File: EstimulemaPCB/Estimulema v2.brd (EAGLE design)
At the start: 151 x 162 mm, 159 parts, among them IC3 74AC14N, IC4 ISO7240S, J1 JUMPERS12MM, J2 J15MM, J3 J_7MM, J4 JUMPERS5MM, J5 JUMPERS7MM, J6 J7MM, K2 HC-06, Q17 TIP48, Q18 TIP50, Q19 TIP50_TH, Q20 TIP50, Q21 TIP50_TH, Q22 TIP48, Q23 TIP48_TH, Q24 TIP48_TH, Q33 TIP48, Q34 TIP50, Q35 TIP50_TH, Q36 TIP50, Q37 TIP50_TH, Q38 TIP48, Q39 TIP48_TH, Q40 TIP48_TH, X1HV+ CONECTOR_5.08, X2+15- CONECTOR_5.08, X3HV- CONECTOR_5.08

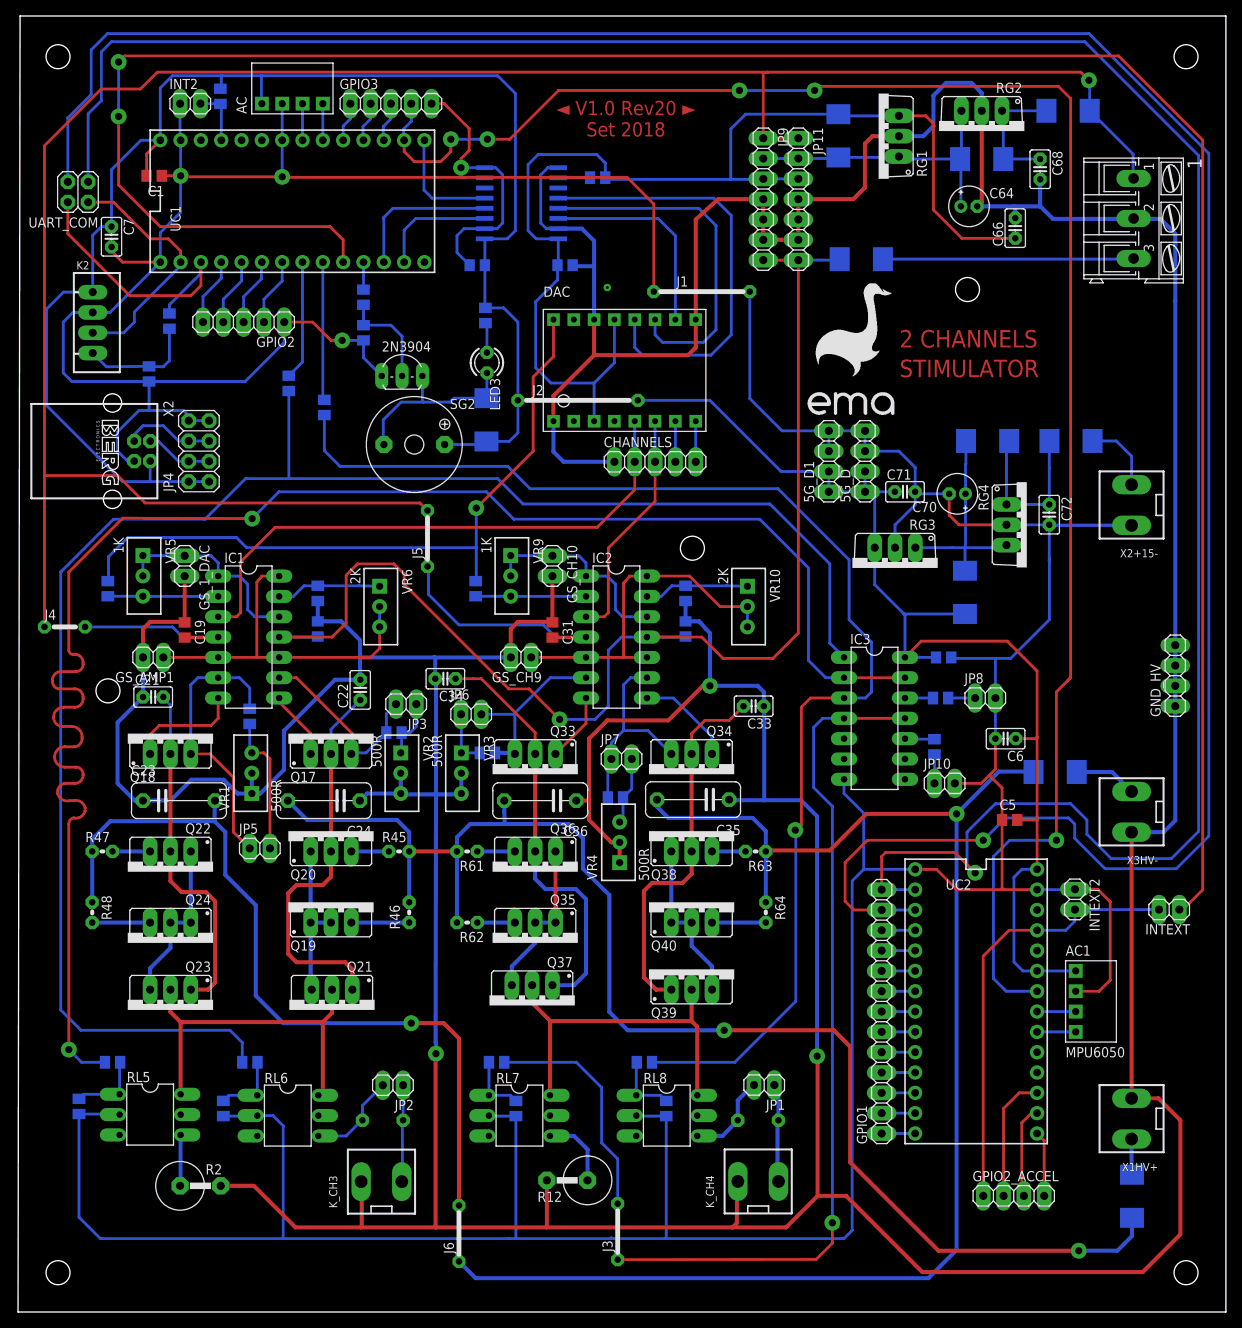
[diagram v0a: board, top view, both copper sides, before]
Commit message: New version eagle 9.2
arreglando algunas cosas
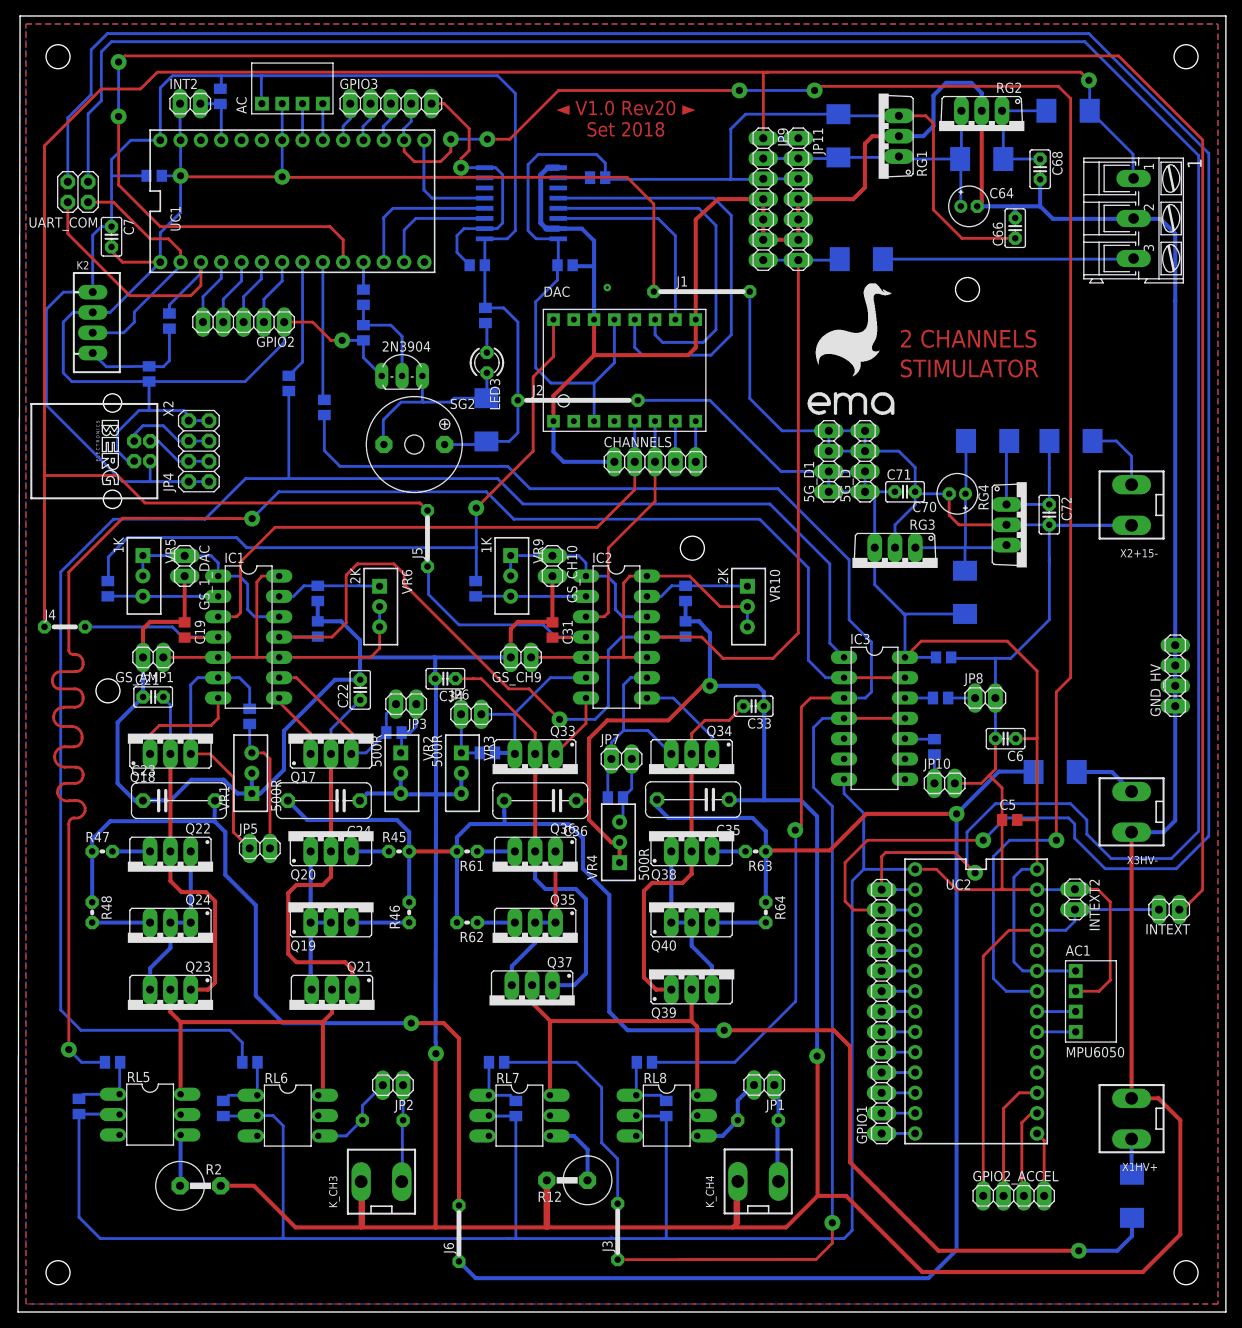
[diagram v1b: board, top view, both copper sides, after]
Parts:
- flipped C1 to the bottom, turned to 0 degrees
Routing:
- net GND_D: track 665.0 -> 669.5 mm
- net +5_D: track 338.5 -> 343.0 mm
- net +8_HV: track 38.6 -> 37.5 mm
- net N$73: track 24.4 -> 23.6 mm
- net N$158: track 22.9 -> 22.3 mm
- net N$145: track 21.1 -> 20.5 mm
- net N$111: track 44.1 -> 43.6 mm
- added copper zone on layer 1, net GND_HV
- added copper zone on layer 16, net GND_HV

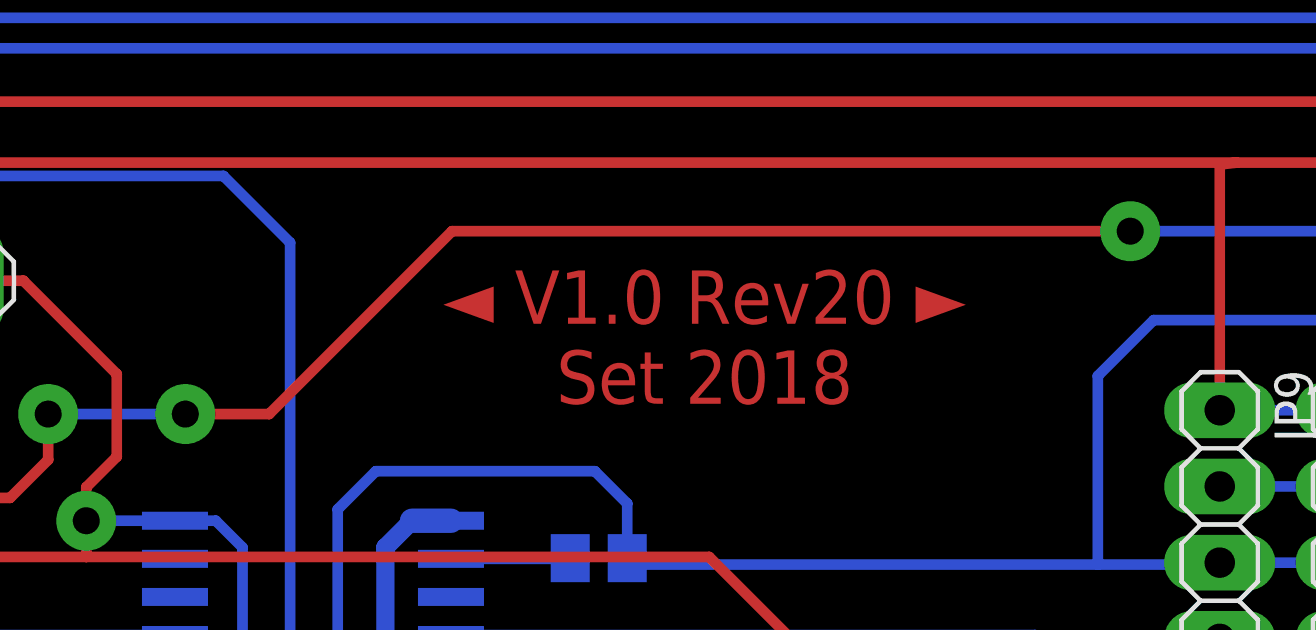
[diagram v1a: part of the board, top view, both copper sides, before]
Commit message: last version pcb file
ultima version pcb
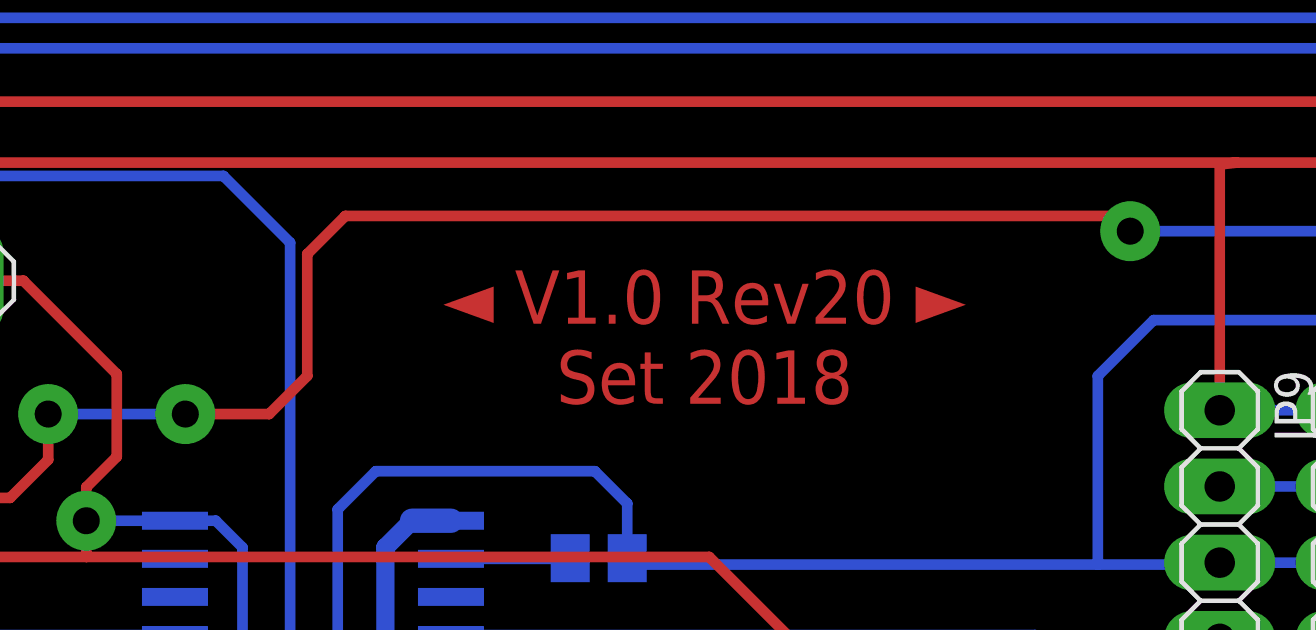
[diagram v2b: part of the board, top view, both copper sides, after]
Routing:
- net GPIO5: track 219.2 -> 222.0 mm
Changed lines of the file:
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@@
 <drawing>
 <settings>
-<setting alwaysvectorfont="yes"/>
+<setting alwaysvectorfont="no"/>
 <setting verticaltext="up"/>
 </settings>
@@
 </layers>
 <board>
-<fusionsync huburn="a.cGVyc29uYWw6dWUyOGM0MjA1" projecturn="a.cGVyc29uYWw6dWUyOGM0MjA1IzIwMTcxMjI2MTA5OTE4NzUx" f3durn="urn:adsk.wipprod:dm.lineage:a3TV6h6ST9ayQOR__9NI6g" pcbguid="653ef68f-6985-4a81-9d55-14a2d5d2a77c" lastpulledtime="" lastsyncedchangeguid="1821962e-2547-75dc-39ca-bfed1a03af76"/>
+<fusionsync huburn="a.cGVyc29uYWw6dWUyOGM0MjA1" projecturn="a.cGVyc29uYWw6dWUyOGM0MjA1IzIwMTcxMjI2MTA5OTE4NzUx" f3durn="urn:adsk.wipprod:dm.lineage:a3TV6h6ST9ayQOR__9NI6g" pcbguid="653ef68f-6985-4a81-9d55-14a2d5d2a77c" lastpulledtime="" lastsyncedchangeguid="752f2832-0191-109f-3336-40c44a7aafc6"/>
 <plain>
 <wire x1="1.016" y1="50" x2="152" y2="50" width="0" layer="20"/>
@@
 <wire x1="55.118" y1="196.596" x2="59.69" y2="196.596" width="0.3556" layer="16"/>
 <via x="59.69" y="196.596" extent="1-16" drill="0.9" diameter="2" shape="square"/>
-<wire x1="59.69" y1="196.596" x2="62.484" y2="196.596" width="0.3556" layer="1"/>
+<wire x1="62.484" y1="196.596" x2="59.69" y2="196.596" width="0.3556" layer="1"/>
 <via x="91.186" y="202.692" extent="1-16" drill="0.9" diameter="2" shape="square"/>
 <wire x1="91.186" y1="202.692" x2="100.584" y2="202.692" width="0.3556" layer="16"/>
@@
 <wire x1="124.5362" y1="90.0938" x2="122.936" y2="91.694" width="0.3556" layer="16"/>
 <wire x1="122.936" y1="106.934" x2="122.936" y2="91.694" width="0.3556" layer="16"/>
-<wire x1="62.484" y1="196.596" x2="68.58" y2="202.692" width="0.3556" layer="1"/>
-<wire x1="68.58" y1="202.692" x2="91.186" y2="202.692" width="0.3556" layer="1"/>
 <wire x1="100.584" y1="202.692" x2="101.092" y2="203.2" width="0.3556" layer="1"/>
 <wire x1="124.968" y1="108.966" x2="122.936" y2="106.934" width="0.3556" layer="16"/>
@@
 <wire x1="101.092" y1="203.2" x2="131.064" y2="203.2" width="0.3556" layer="1"/>
 <wire x1="130.81" y1="127.508" x2="132.588" y2="129.286" width="0.3556" layer="1"/>
+<wire x1="65.024" y1="203.2" x2="63.754" y2="201.93" width="0.3556" layer="1"/>
+<wire x1="63.754" y1="201.93" x2="63.754" y2="197.866" width="0.3556" layer="1"/>
+<wire x1="63.754" y1="197.866" x2="62.484" y2="196.596" width="0.3556" layer="1"/>
+<wire x1="91.186" y1="202.692" x2="90.678" y2="203.2" width="0.3556" layer="1"/>
+<wire x1="90.678" y1="203.2" x2="65.024" y2="203.2" width="0.3556" layer="1"/>
 </signal>
 <signal name="GPIO6" class="2">
